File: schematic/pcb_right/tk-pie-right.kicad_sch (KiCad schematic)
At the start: 35 parts, among them IC1 PCA9539PW,118, J1 NiceView, J2 Battery Connector, U3 SN74LVC1T45DCK

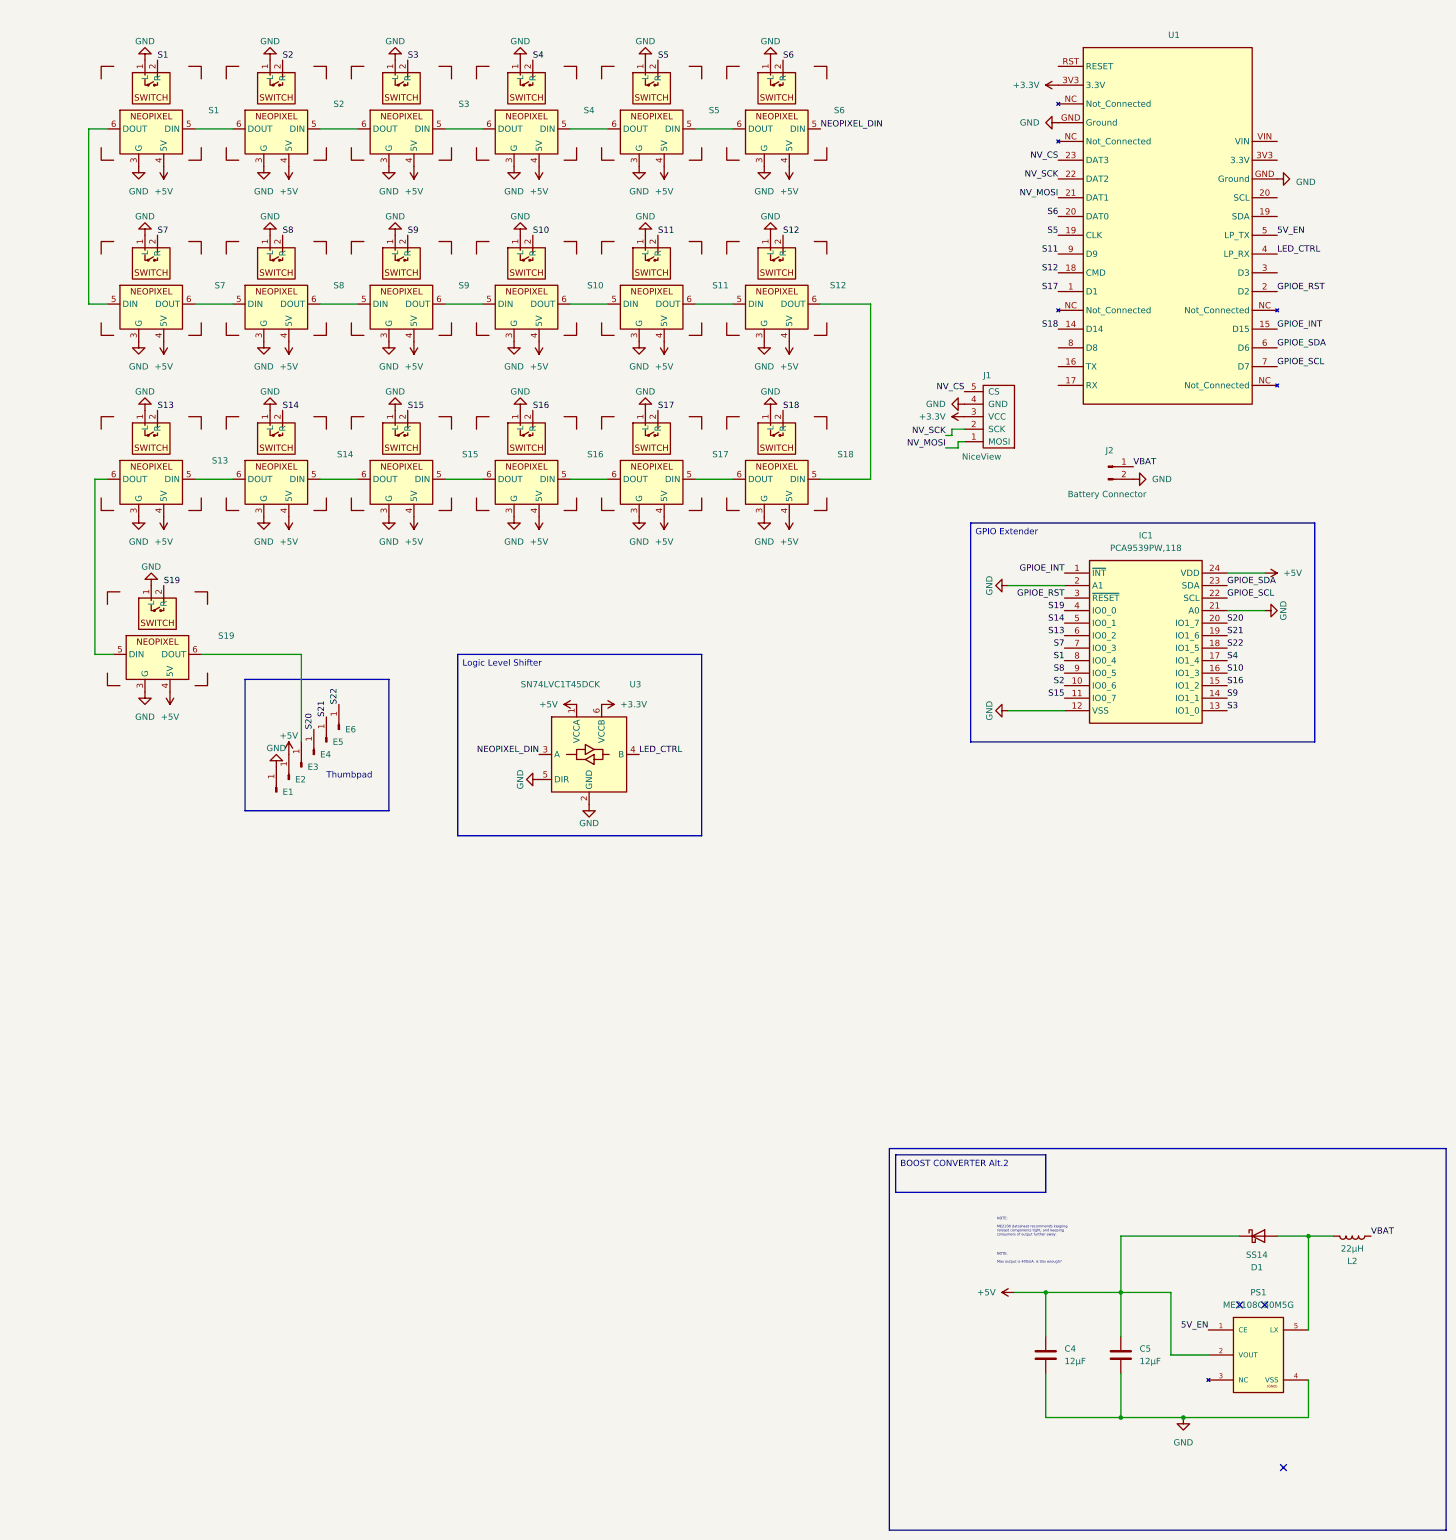
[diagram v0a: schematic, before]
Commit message: RIGHT PCB ???? TRACES VIAS!!!!
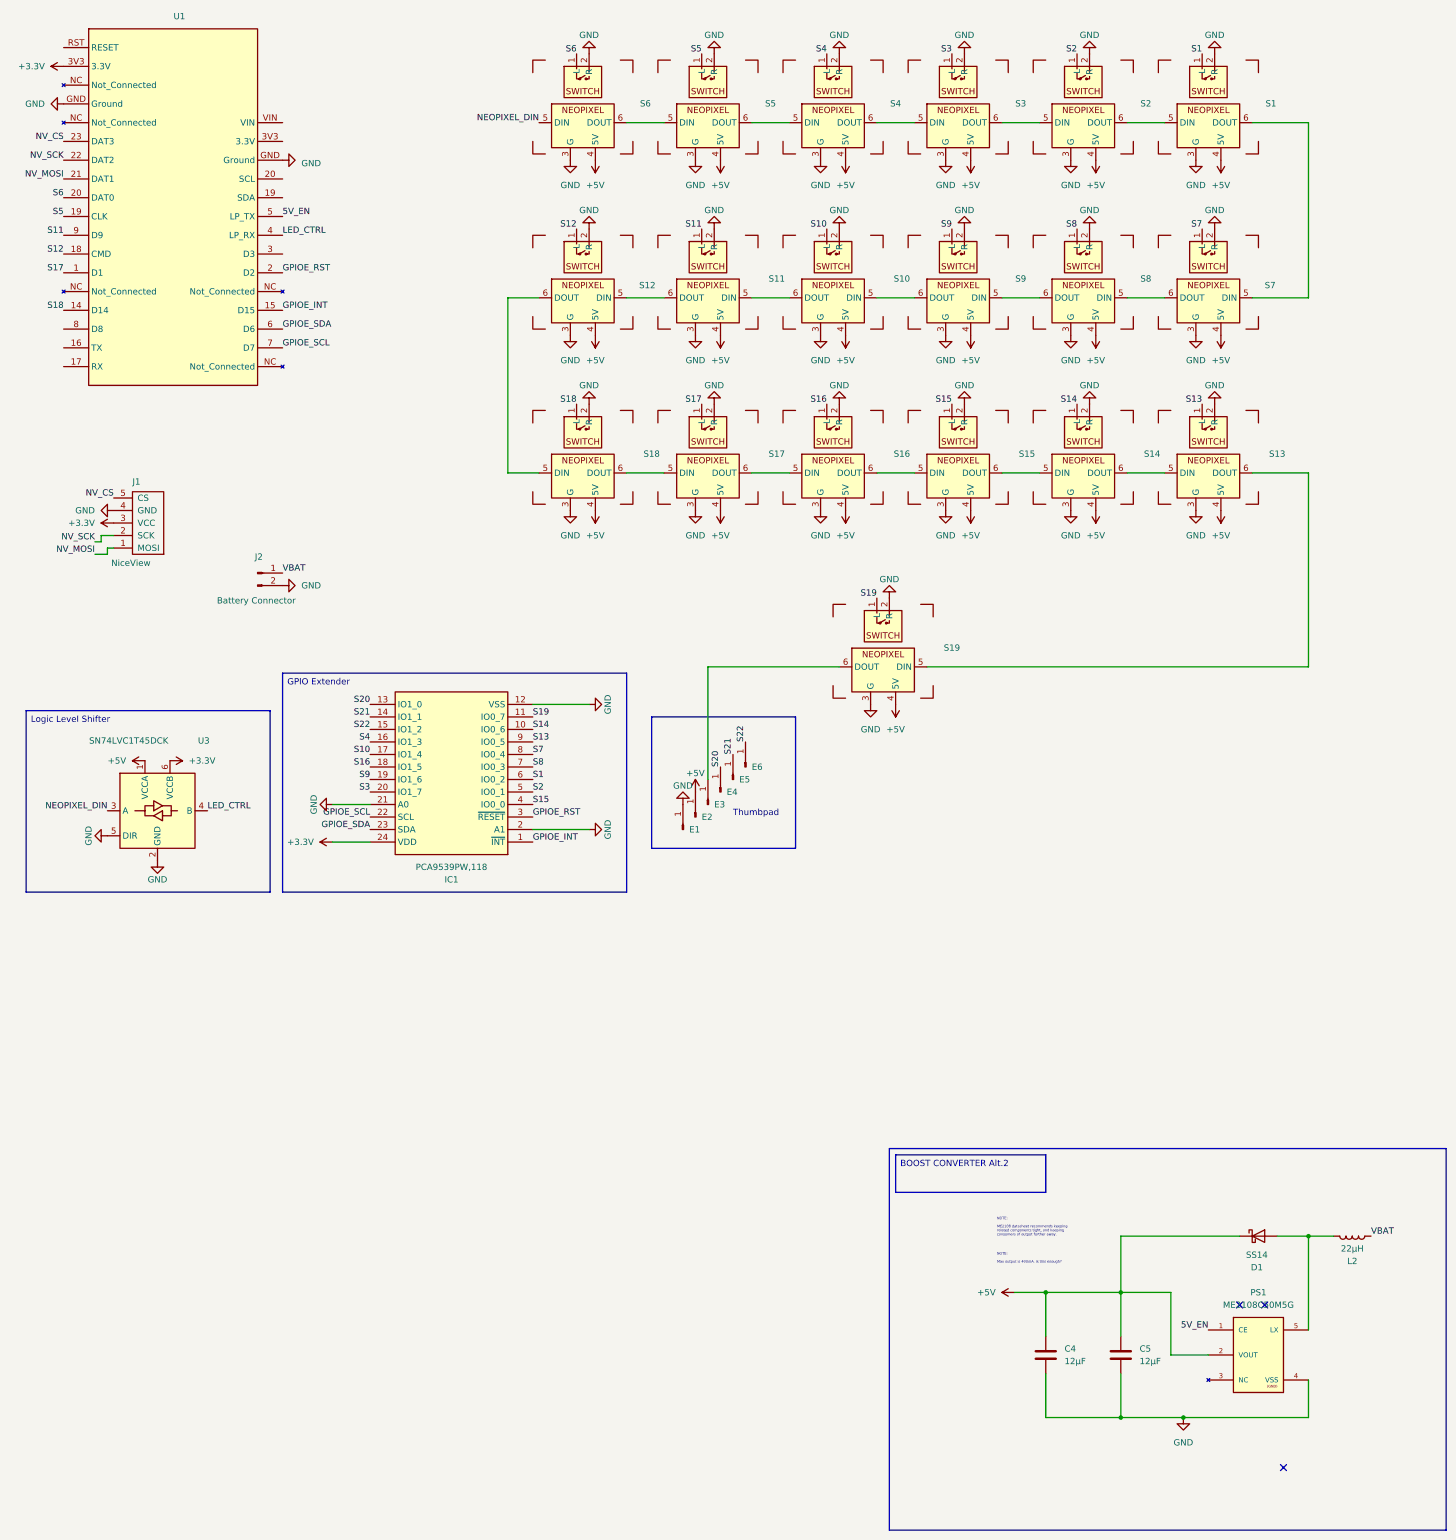
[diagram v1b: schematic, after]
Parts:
- S1, S13, S4, S5, S6: value MX_SW_SOCKET_LED -> MX_SW_SOCKET_RGB_REV; footprint Footprints:MX_SW_SOCKET_LED -> Footprints:MX_SW_SOCKET_LED_REV; symbol library:MX_SW_SOCKET_RGB -> library:MX_SW_SOCKET_RGB_REV
- S10, S11, S12, S19, S7, S8, S9: value MX_SW_SOCKET_RGB_REV -> MX_SW_SOCKET_LED; footprint Footprints:MX_SW_SOCKET_LED_REV -> Footprints:MX_SW_SOCKET_LED; symbol library:MX_SW_SOCKET_RGB_REV -> library:MX_SW_SOCKET_RGB
- S14, S15, S16, S17, S18, S2, S3: value ~ -> MX_SW_SOCKET_RGB_REV; footprint Footprints:MX_SW_SOCKET_LED -> Footprints:MX_SW_SOCKET_LED_REV; symbol library:MX_SW_SOCKET_RGB -> library:MX_SW_SOCKET_RGB_REV
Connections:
- net +3.3V: now also IC1.24 (VDD)
- net +5V: no longer IC1.24 (VDD)
- net GND: now also S1.2 (R), S10.2 (R), S11.2 (R), S12.2 (R), S13.2 (R), S14.2 (R), S15.2 (R), S16.2 (R), S17.2 (R), S18.2 (R), S19.2 (R), S2.2 (R), S3.2 (R), S4.2 (R), S5.2 (R), S6.2 (R), S7.2 (R), S8.2 (R), S9.2 (R); no longer S1.1 (L), S10.1 (L), S11.1 (L), S12.1 (L), S13.1 (L), S14.1 (L), S15.1 (L), S16.1 (L), S17.1 (L), S18.1 (L), S19.1 (L), S2.1 (L), S3.1 (L), S4.1 (L), S5.1 (L), S6.1 (L), S7.1 (L), S8.1 (L), S9.1 (L)
- net S1: now also IC1.6 (IO0_2), S1.1 (L); no longer IC1.8 (IO0_4), S1.2 (R)
- net S10: now also IC1.17 (IO1_4), S10.1 (L); no longer IC1.16 (IO1_3), S10.2 (R)
- net S11: now also S11.1 (L); no longer S11.2 (R)
- net S12: now also S12.1 (L); no longer S12.2 (R)
- net S13: now also IC1.9 (IO0_5), S13.1 (L); no longer IC1.6 (IO0_2), S13.2 (R)
- net S14: now also IC1.10 (IO0_6), S14.1 (L); no longer IC1.5 (IO0_1), S14.2 (R)
- net S15: now also IC1.4 (IO0_0), S15.1 (L); no longer IC1.11 (IO0_7), S15.2 (R)
- net S16: now also IC1.18 (IO1_5), S16.1 (L); no longer IC1.15 (IO1_2), S16.2 (R)
- net S17: now also S17.1 (L); no longer S17.2 (R)
- net S18: now also S18.1 (L); no longer S18.2 (R)
- net S19: now also IC1.11 (IO0_7), S19.1 (L); no longer IC1.4 (IO0_0), S19.2 (R)
- net S2: now also IC1.5 (IO0_1), S2.1 (L); no longer IC1.10 (IO0_6), S2.2 (R)
- net S20: now also IC1.13 (IO1_0); no longer IC1.20 (IO1_7)
- net S21: now also IC1.14 (IO1_1); no longer IC1.19 (IO1_6)
- net S22: now also IC1.15 (IO1_2); no longer IC1.18 (IO1_5)
- net S3: now also IC1.20 (IO1_7), S3.1 (L); no longer IC1.13 (IO1_0), S3.2 (R)
- net S4: now also IC1.16 (IO1_3), S4.1 (L); no longer IC1.17 (IO1_4), S4.2 (R)
- net S5: now also S5.1 (L); no longer S5.2 (R)
- net S6: now also S6.1 (L); no longer S6.2 (R)
- net S7: now also IC1.8 (IO0_4), S7.1 (L); no longer IC1.7 (IO0_3), S7.2 (R)
- net S8: now also IC1.7 (IO0_3), S8.1 (L); no longer IC1.9 (IO0_5), S8.2 (R)
- net S9: now also IC1.19 (IO1_6), S9.1 (L); no longer IC1.14 (IO1_1), S9.2 (R)
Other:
- moved on the sheet: E1, E2, E3, E4, E5, E6, IC1, J1, J2, S1, S10, S11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
